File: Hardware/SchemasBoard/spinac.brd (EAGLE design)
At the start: 49.9 x 22.9 mm, 28 parts, among them IC1 LNK304, IC2 MCP1703DB, IC4 DS1820, K1 G5L, T1 BC846

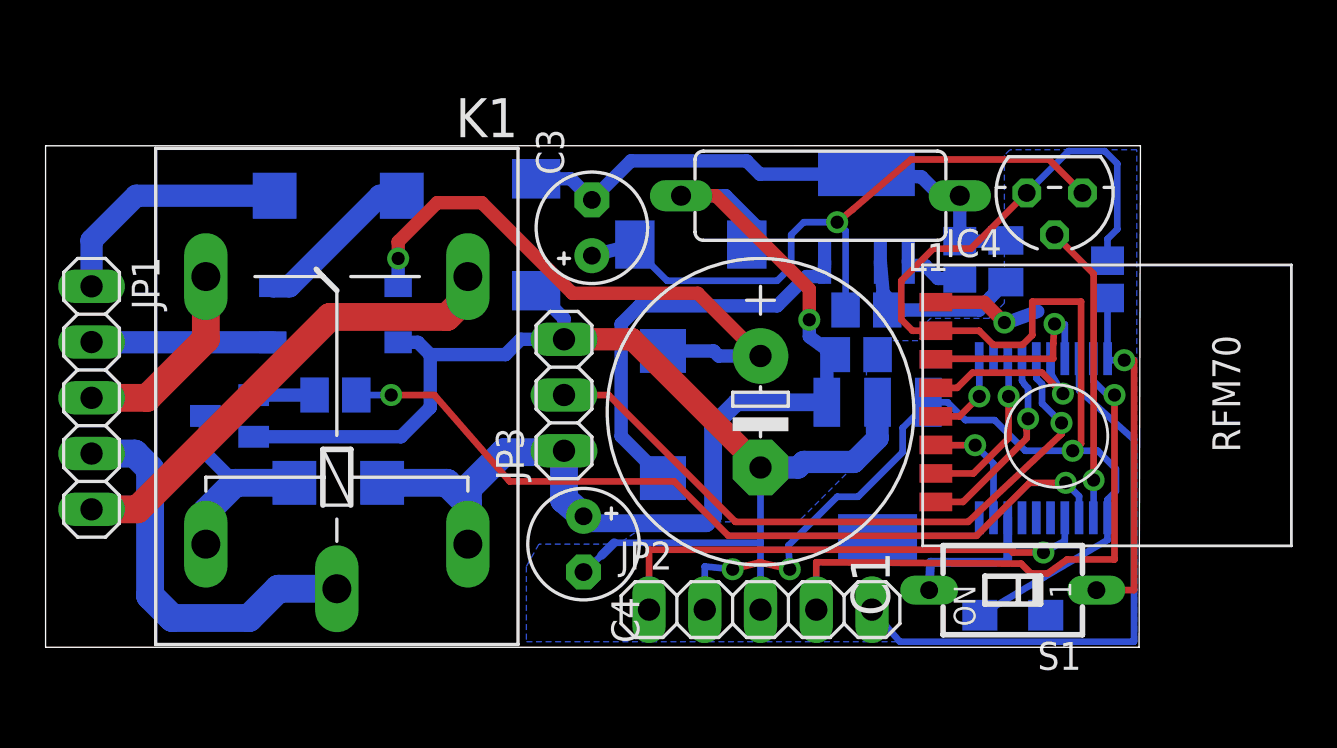
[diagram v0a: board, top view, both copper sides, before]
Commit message: aaa
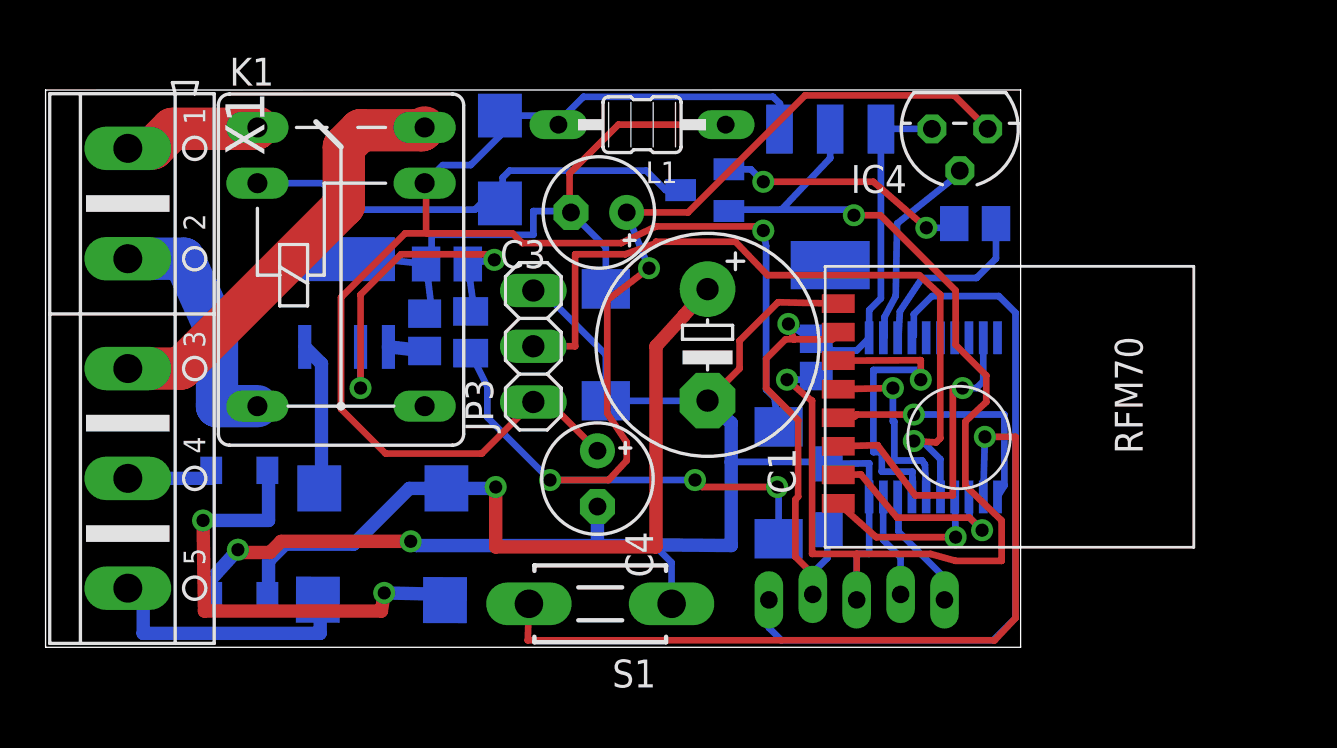
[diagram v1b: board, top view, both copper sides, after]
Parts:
- removed JP1, JP2: (no value), pinhead:1X05
- removed R7: 2 K, resistor:M2012
- added U$3: PROGRAMMINGHEADERDIP, rfm70:PROGHEADER
- added X1: (no value), con-ptr500:AK500/5
- C1: device resistor:E5-13 -> resistor:E5-10,5
- K1: value G5L -> FRS1B; device relay:G5LE -> relay:FRS1B
- L1: value BC12 -> MMICC7; device inductors:BC12 -> inductors:MMICC7
- S1: value (none) -> DTS-3; device switch-dil:SD4-01 -> switch-tact:DTS-3
- moved R5 30.2 mm to (42.4, 19.3)
- moved R4 25.5 mm to (18.3, 17.5), turned to 0 degrees
- moved C2 24.6 mm to (17.3, 14.4)
- moved IC1 24.0 mm to (13.7, 15.7)
- moved T1 24.0 mm to (30.0, 20.8)
- moved S1 18.8 mm to (25.3, 1.98), turned to 180 degrees
- moved R2 18.5 mm to (15.3, 2.16), turned to 180.2 degrees
- moved R3 18.1 mm to (19.4, 14.4), turned to 90 degrees
- moved D1 16.5 mm to (20.7, 22.2), turned to 270 degrees
- moved C5 13.7 mm to (35.1, 13.2)
- moved R1 13.2 mm to (15.4, 7.24), turned to 0 degrees
- moved IC2 12.6 mm to (35.8, 20.5)
- moved D4 11.6 mm to (33.4, 7.49), turned to 90 degrees
- moved B1 10.9 mm to (8.83, 5.21), turned to 0 degrees
- moved C6 10.0 mm to (35.6, 6.86), turned to 90 degrees
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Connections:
- net GND: now also U$3.GND; no longer JP2.3, R7.1
- net N$17: now also U$3.VDD; no longer JP2.2
- net N$18: now also U$3.PGD; no longer JP2.4
- net N$19: now also U$3.PGC; no longer JP2.5
- net N$24: now also X1.1; no longer JP1.3
- net N$25: now also U$3.MCLR; no longer JP2.1
- net N$26: no longer R7.2
- net N$36: now also X1.5; no longer JP1.1
- net N$4: now also X1.4; no longer JP1.2
- net N$5: now also U$2.12; no longer U$2.8
- net N$7: now also K1.P@, X1.2; no longer JP1.5, K1.S
- net N$8: now also K1.S, X1.3; no longer JP1.4, K1.P
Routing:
- net GND: track 77.2 -> 122.0 mm, vias 2 -> 4
- net N$17: track 73.1 -> 36.8 mm, vias 3 -> 1
- net N$5: track 6.82 -> 36.7 mm, vias 0 -> 1
- net N$35: track 38.0 -> 8.37 mm, vias 2 -> 0
- net N$9: track 31.0 -> 55.9 mm, vias 1 -> 4
- net N$18: track 26.0 -> 4.78 mm, vias 1 -> 0
- net N$19: track 26.6 -> 5.58 mm
- net N$26: track 53.2 -> 71.9 mm
- net N$3: track 7.59 -> 21.4 mm, vias 0 -> 2
- net N$14: track 9.65 -> 21.4 mm
- net N$1: track 18.6 -> 7.54 mm
- net N$7: track 22.1 -> 11.4 mm
- net N$25: track 23.0 -> 33.5 mm, vias 1 -> 0
- net N$2: track 26.7 -> 36.0 mm
- net N$23: track 5.45 -> 14.8 mm
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- removed copper zone on layer 16, net GND
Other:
- board size 49.9 x 22.9 mm -> 44.4 x 25.4 mm

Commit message: a
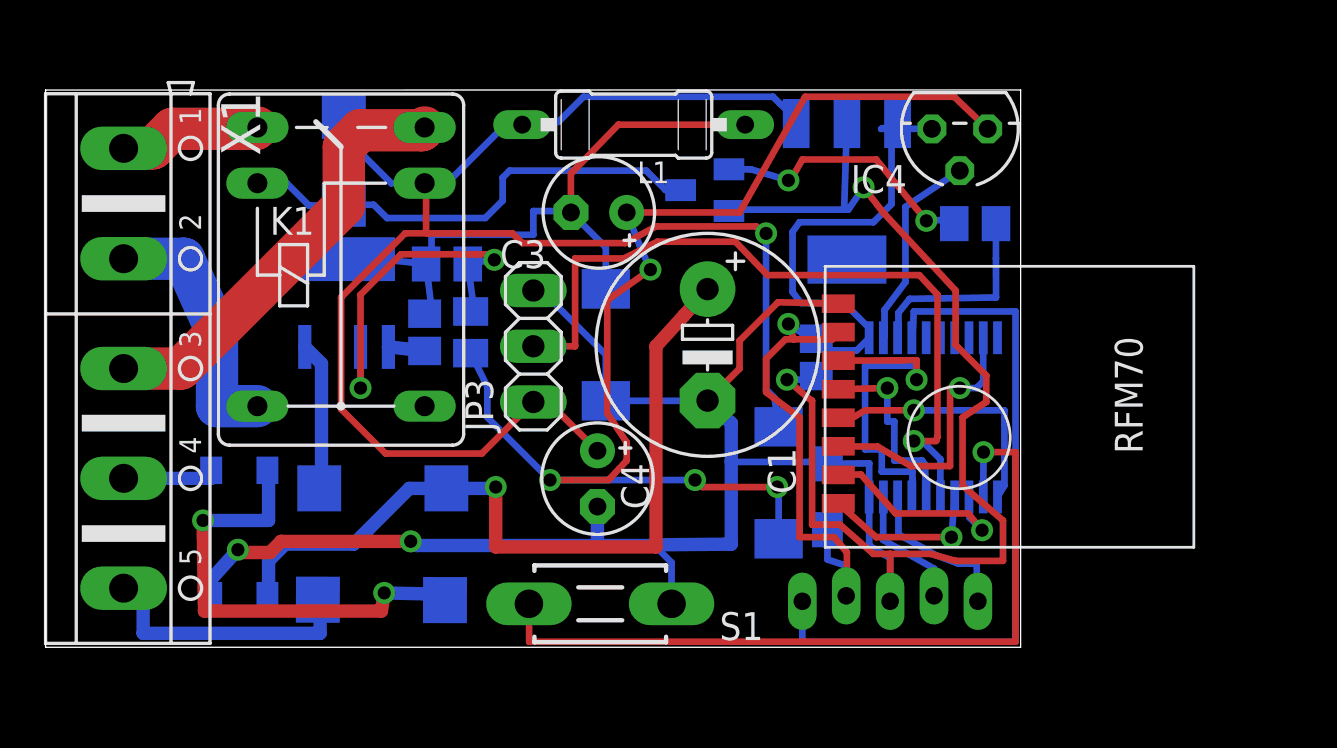
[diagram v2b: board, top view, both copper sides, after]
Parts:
- L1: value MMICC7 -> MICC10; device inductors:MMICC7 -> inductors:MICC10
- moved D1 7.11 mm to (13.6, 22.2)
- moved U$3 1.53 mm to (38.5, 2.10)
- moved IC2 0.80 mm to (36.5, 20.8)
- moved L1 0.38 mm to (26.8, 23.8)
- moved X1 0.19 mm to (3.56, 12.7)
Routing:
- net N$17: track 36.8 -> 46.1 mm
- net N$26: track 71.9 -> 76.8 mm
- net N$23: track 14.8 -> 12.5 mm
- net N$19: track 5.58 -> 7.33 mm
- net N$18: track 4.78 -> 5.87 mm
- net N$15: track 11.4 -> 12.4 mm
- net N$25: track 33.5 -> 32.4 mm
- net N$13: track 29.0 -> 30.0 mm, vias 1 -> 0
- net N$9: track 55.9 -> 56.8 mm
- net N$35: track 8.37 -> 9.27 mm
- net N$16: track 14.8 -> 15.6 mm
- net N$5: track 36.7 -> 36.0 mm

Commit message: New version
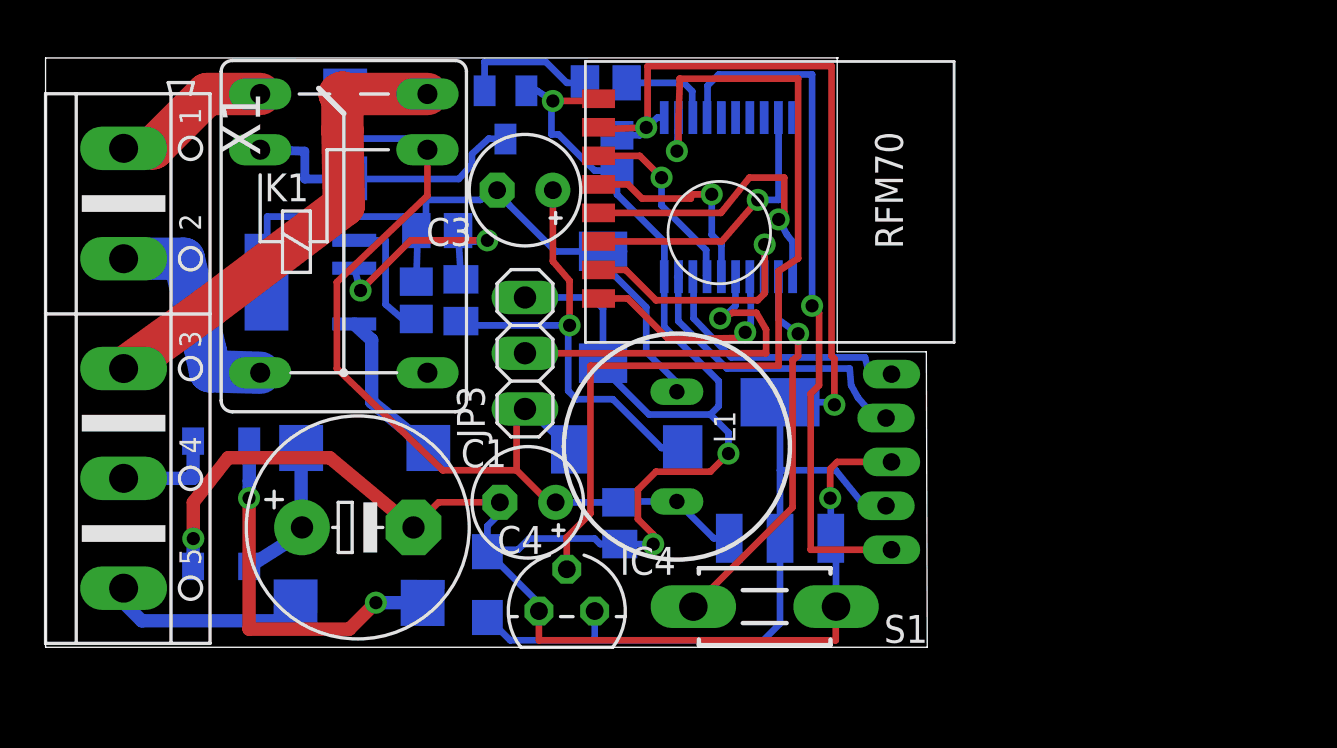
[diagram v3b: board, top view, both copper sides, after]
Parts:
- removed IC2: MCP1703DB, linear:SOT223
- added IC3: MC33269ST-3.3T3, linear:SOT223
- added R6: 1 K, resistor:M2012
- L1: value MICC10 -> 680uH; device inductors:MICC10 -> inductor-neosid:BS11
- moved IC4 28.3 mm to (23.7, 1.65), turned to 0 degrees
- moved R5 18.0 mm to (25.5, 25.7)
- moved C1 18.0 mm to (14.2, 5.46), turned to 0 degrees
- moved C6 16.0 mm to (20.1, 2.86)
- moved L1 14.8 mm to (28.8, 9.14), turned to 270 degrees
- moved U$1 14.4 mm to (39.5, 24.9)
- moved U$2 13.7 mm to (31.1, 20.5)
- moved C5 13.0 mm to (26.0, 22.5)
- moved T1 9.71 mm to (21.0, 24.3), turned to 180 degrees
- moved S1 7.49 mm to (32.8, 1.85)
- moved D4 7.09 mm to (26.5, 9.02), turned to 0 degrees
- moved U$3 6.35 mm to (38.5, 8.45), turned to 90 degrees
- moved C3 3.52 mm to (21.8, 20.8)
- moved C4 3.35 mm to (22.0, 6.60), turned to 180 degrees
- moved R1 2.02 mm to (14.5, 9.08), turned to 180 degrees
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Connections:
- removed net N$17: C5.2, C6.+, IC2.3, IC4.3, U$1.VDD, U$2.1, U$3.VDD
- new net N$28: C5.2, C6.+, IC3.2, IC3.4, IC4.3, U$1.VDD, U$2.1, U$3.VDD
- net GND: now also IC3.1, IC4.1, R6.1; no longer IC2.2
- net N$26: now also IC3.3, R6.2; no longer IC2.1
- net N$9: no longer IC4.1
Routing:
- net N$28: track 0.09 -> 65.0 mm, vias 0 -> 2
- net N$17: track 46.1 -> 0.00 mm, vias 1 -> 0
- net N$9: track 56.8 -> 20.8 mm, vias 4 -> 1
- net N$6: track 9.28 -> 42.2 mm, vias 0 -> 1
- net N$26: track 76.8 -> 44.7 mm, vias 1 -> 0
- net N$2: track 36.0 -> 7.07 mm, vias 1 -> 0
- net N$5: track 36.0 -> 17.5 mm
- net N$32: track 34.6 -> 16.9 mm
- net GND: track 122.1 -> 104.8 mm, vias 4 -> 5
- net N$18: track 5.87 -> 13.8 mm
- net N$14: track 21.8 -> 14.5 mm
- net N$16: track 15.6 -> 8.65 mm
- net N$15: track 12.4 -> 6.28 mm, vias 2 -> 0
- net N$19: track 7.33 -> 12.3 mm
- net N$35: track 9.27 -> 4.35 mm
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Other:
- board size 44.4 x 25.4 mm -> 40.2 x 26.9 mm

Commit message: hf
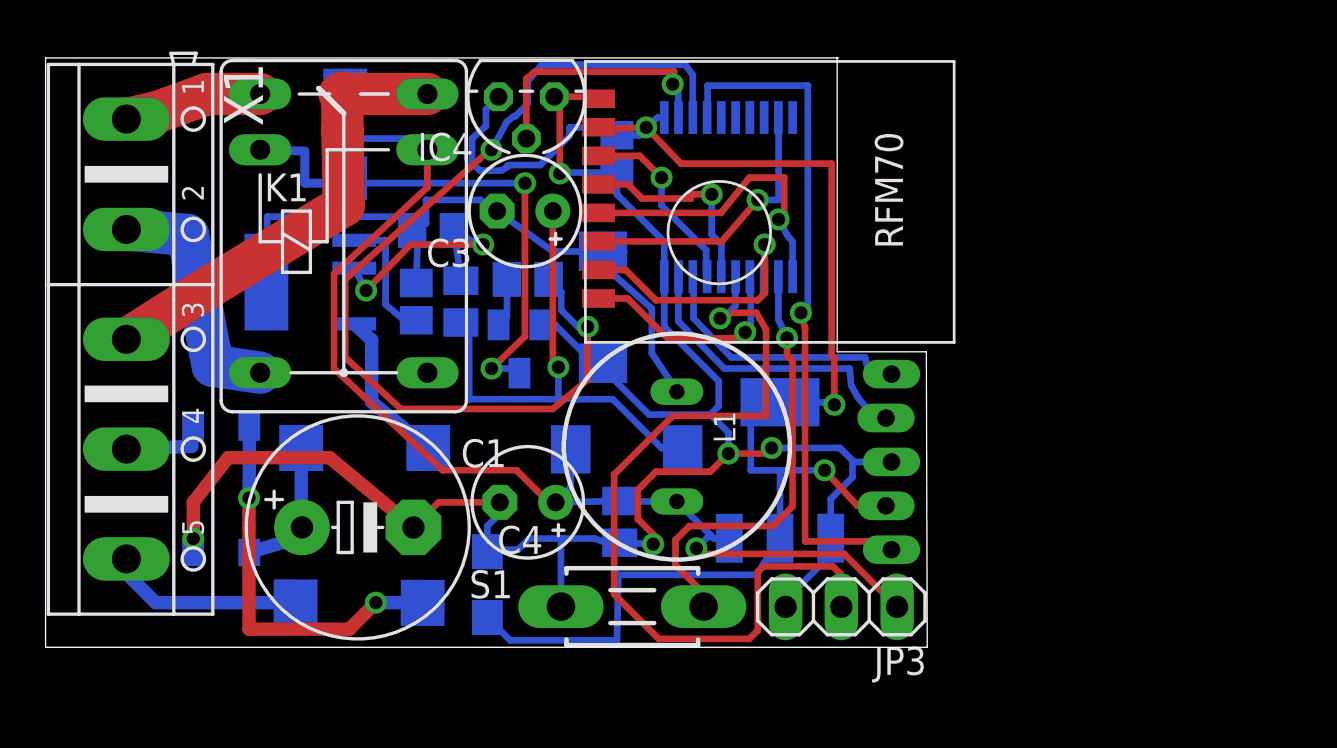
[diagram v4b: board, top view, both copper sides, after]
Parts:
- moved IC4 23.5 mm to (21.9, 25.1), turned to 180 degrees
- moved JP3 18.5 mm to (36.3, 1.84), turned to 180 degrees
- moved T1 10.7 mm to (21.6, 13.6)
- moved R5 9.63 mm to (22.0, 16.8)
- moved S1 6.03 mm to (26.7, 1.85), turned to 0 degrees
- moved X1 1.34 mm to (3.68, 14.0)
- moved C3 0.95 mm to (21.8, 19.9)
- moved B1 0.64 mm to (8.00, 7.18)
- moved R4 0.19 mm to (17.7, 19.0)
- moved C2 0.06 mm to (16.9, 15.7)
- moved R3 0.06 mm to (18.9, 15.7)
- moved R6 0.06 mm to (26.2, 5.71)
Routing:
- net N$35: track 4.35 -> 44.4 mm, vias 0 -> 2
- net N$6: track 42.2 -> 11.9 mm
- net N$32: track 16.9 -> 38.0 mm
- net GND: track 104.8 -> 89.7 mm
- net N$14: track 14.5 -> 24.4 mm, vias 0 -> 2
- net N$26: track 44.7 -> 52.9 mm, vias 0 -> 1
- net N$28: track 65.0 -> 70.8 mm, vias 2 -> 3
- net N$15: track 6.28 -> 2.23 mm
- net N$5: track 17.5 -> 20.2 mm
- net N$9: track 20.8 -> 23.5 mm
- net N$8: track 21.8 -> 20.8 mm
- net N$4: track 4.86 -> 3.85 mm
- net N$24: track 7.25 -> 6.28 mm
- net N$13: track 33.3 -> 32.5 mm
- net N$7: track 10.3 -> 11.1 mm
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
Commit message: fixed power supply 22 uF C3 and differend FW diode
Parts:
- C3: value 10uF / 16 V -> 22uF / 16 V
- D3: value (none) -> UF4007
- D4: value (none) -> 1N4007GP
- L1: value 680uH -> 1mH
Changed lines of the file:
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@@
 <element name="R4" library="resistor" package="M2012" value="2,05 k" x="17.653" y="18.9865" rot="MR0"/>
 <element name="R5" library="resistor" package="M2012" value="1 K" x="21.971" y="16.764" rot="MR180"/>
-<element name="C3" library="resistor" package="E2,5-5" value="10uF / 16 V" x="21.844" y="19.8755" rot="R180"/>
-<element name="L1" library="inductor-neosid" package="BS11" value="680uH" x="28.7655" y="9.144" smashed="yes" rot="R270">
+<element name="C3" library="resistor" package="E2,5-5" value="22uF / 16 V" x="21.844" y="19.8755" rot="R180"/>
+<element name="L1" library="inductor-neosid" package="BS11" value="1mH" x="28.7655" y="9.144" smashed="yes" rot="R270">
 <attribute name="NAME" x="30.4419" y="10.7696" size="0.9906" layer="25" ratio="10" rot="R270"/>
 <attribute name="VALUE" x="29.6926" y="11.9126" size="0.9906" layer="27" ratio="10" rot="R270"/>
@@
 <element name="C5" library="resistor" package="C2012" value="100nF" x="26.035" y="22.479" rot="MR90"/>
 <element name="T1" library="transistor" package="SOT23" value="BC846" x="21.59" y="13.589" rot="MR180"/>
-<element name="D3" library="diode" package="DO214AA" value="" x="25.4" y="15.494" rot="MR270"/>
-<element name="D4" library="diode" package="DO214AA" value="" x="26.4795" y="9.017" rot="MR0"/>
+<element name="D3" library="diode" package="DO214AA" value="UF4007" x="25.4" y="15.494" rot="MR270"/>
+<element name="D4" library="diode" package="DO214AA" value="1N4007GP" x="26.4795" y="9.017" rot="MR0"/>
 <element name="D1" library="diode" package="SMA" value="MBRA340T3" x="13.6525" y="23.368" rot="MR270"/>
 <element name="JP3" library="pinhead" package="1X03" value="" x="36.2585" y="1.8415" rot="R180"/>
